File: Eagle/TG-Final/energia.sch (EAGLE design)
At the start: 25 parts, among them IC2 7805, IC3 AZ1117

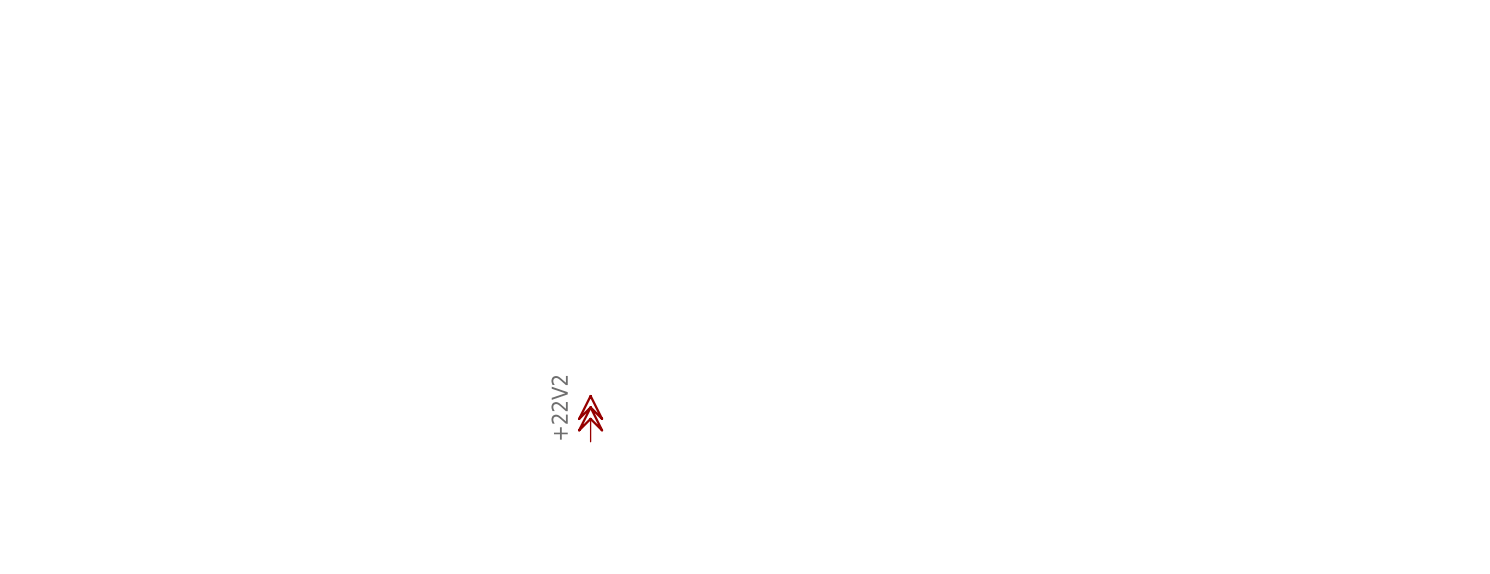
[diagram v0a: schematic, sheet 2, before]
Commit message: Fuente de Potencia
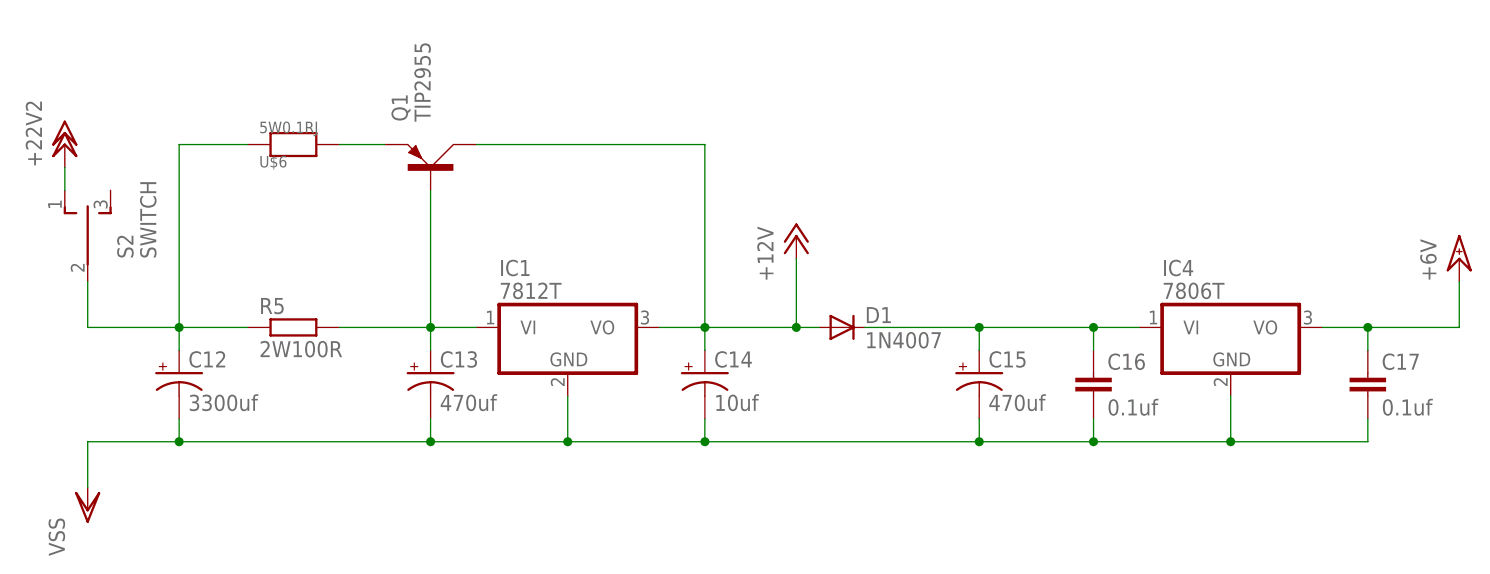
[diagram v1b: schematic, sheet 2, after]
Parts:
- removed R3: 4K7-2W, rcl:R-EU_0411/12
- added C12: 3300uf, rcl:CPOL-USE7.5-18
- added C13, C15: 470uf, rcl:CPOL-USE3.5-8
- added C14: 10uf, rcl:CPOL-USE2.5-5
- added C16, C17: 0.1uf, rcl:C-EU050-024X044
- added D1: 1N4007, diode:1N4004
- added IC1: 7812T, adafruit:7812T
- added IC4: 7806T, adafruit:7806T
- added Q1: TIP2955, transistor-power:TIP2955
- added R5: 2W100R, rcl:R-EU_0411/12
- added S1: SWITCH-2-ESTADOS, aasanchez:TL39YOSWITCH_2_ESTADOS
- added S2: SWITCH, aasanchez:TL39YOSWITCH_2_ESTADOS
- added U$6: 5W0.1RJ, aasanchez:RESISTENCIA5WATT
- added U$9: 10W 5R6J, aasanchez:RESISTENCIA10W
- L1: device rcl:L-EU0207/7 -> rcl:L-EUTFI0307
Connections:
- new net N$1: C1.1, C2.+, L1.1, S1.P
- new net N$13: C15.+, C16.1, D1.C, IC4.VI
- new net N$4: C12.+, R5.1, S2.P, U$6.P$1
- new net N$7: Q1.E, U$6.P$2
- new net N$8: C13.+, IC1.VI, Q1.B, R5.2
- net +11V1: now also S1.O; no longer C1.1, C2.+, L1.1
- net +12V: now also C14.+, D1.A, IC1.VO, Q1.C
- net +22V: now also S2.O
- net +6V: now also C17.1, IC4.VO
- net N$10: now also U$9.P$2; no longer R3.2
- net N$11: now also U$9.P$1; no longer R3.1
- net VSS: now also C12.-, C13.-, C14.-, C15.-, C16.2, C17.2, IC1.GND, IC4.GND
